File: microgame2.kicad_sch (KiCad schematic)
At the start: 17 parts, among them SW9 SW_SPST, U1 ESP32-PICO-D4

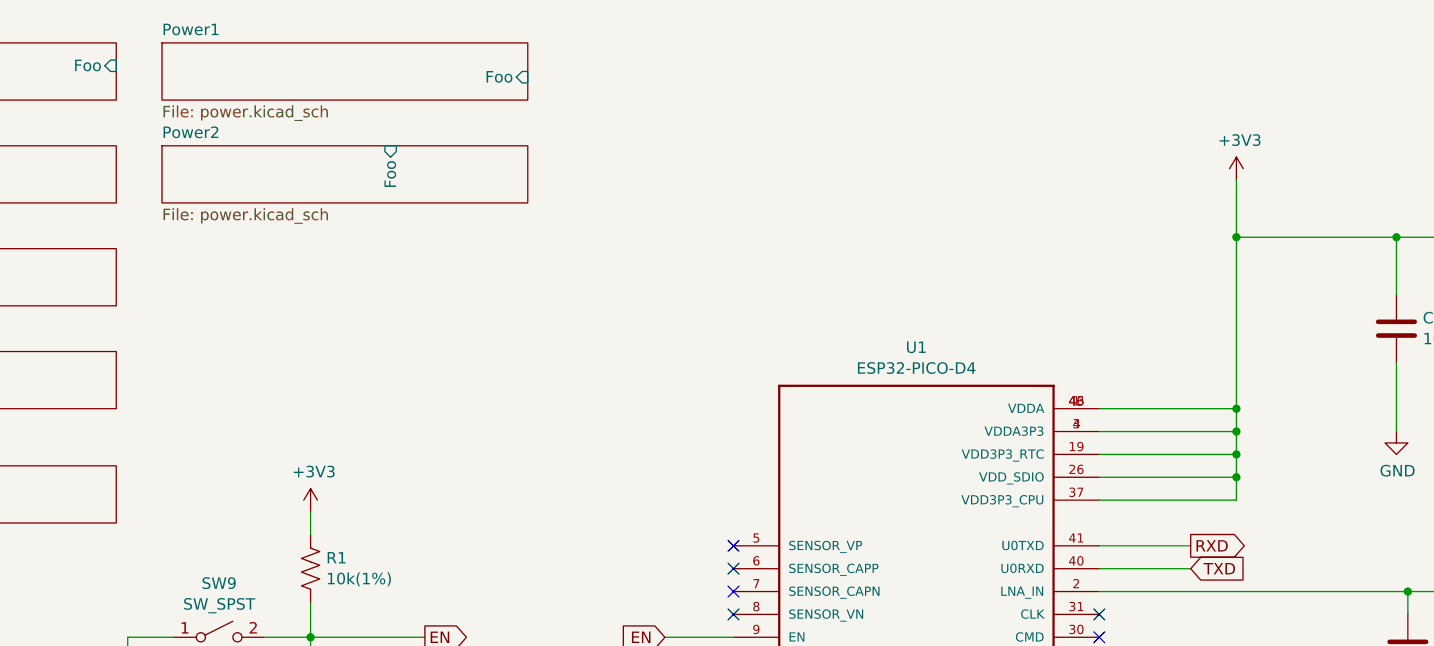
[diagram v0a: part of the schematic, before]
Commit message: reverting
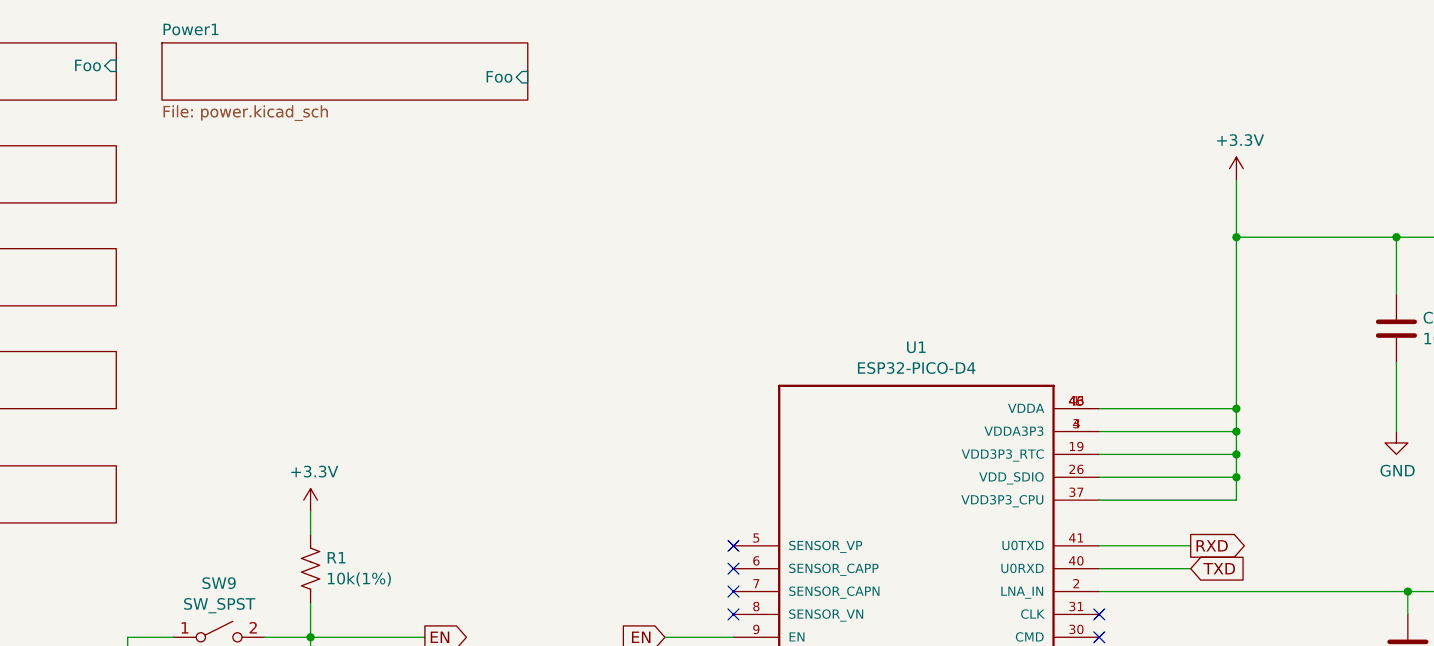
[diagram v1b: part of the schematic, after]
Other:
- removed sheet Power2

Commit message: updating main sch
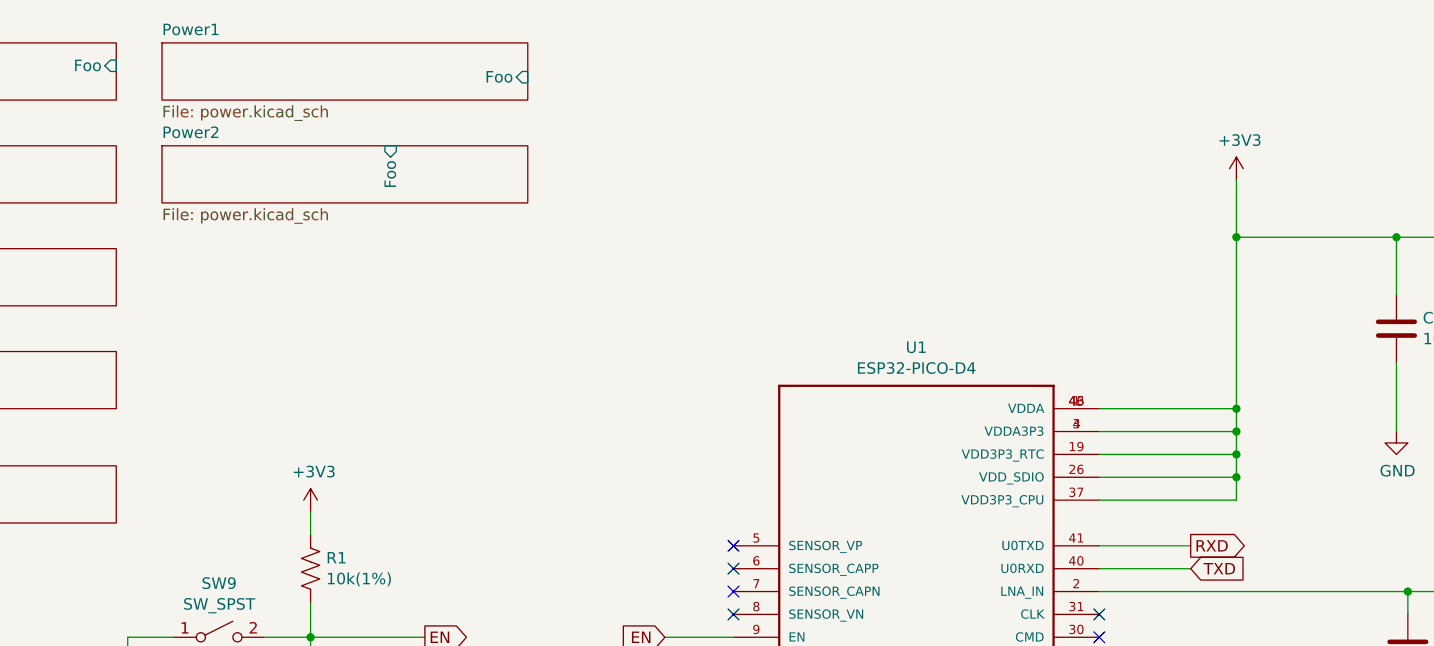
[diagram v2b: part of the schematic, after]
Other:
- added sheet Power2 (power.kicad_sch)
